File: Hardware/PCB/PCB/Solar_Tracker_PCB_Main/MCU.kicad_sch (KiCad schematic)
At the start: 16 parts, among them IC1 ESP32-S3-WROOM-1-N4R8, IC5 LM1117MPX-3.3_NOPB, J2 USB4940-00-A, J3 1729076, J4 1977223-1, J5 1977223-1

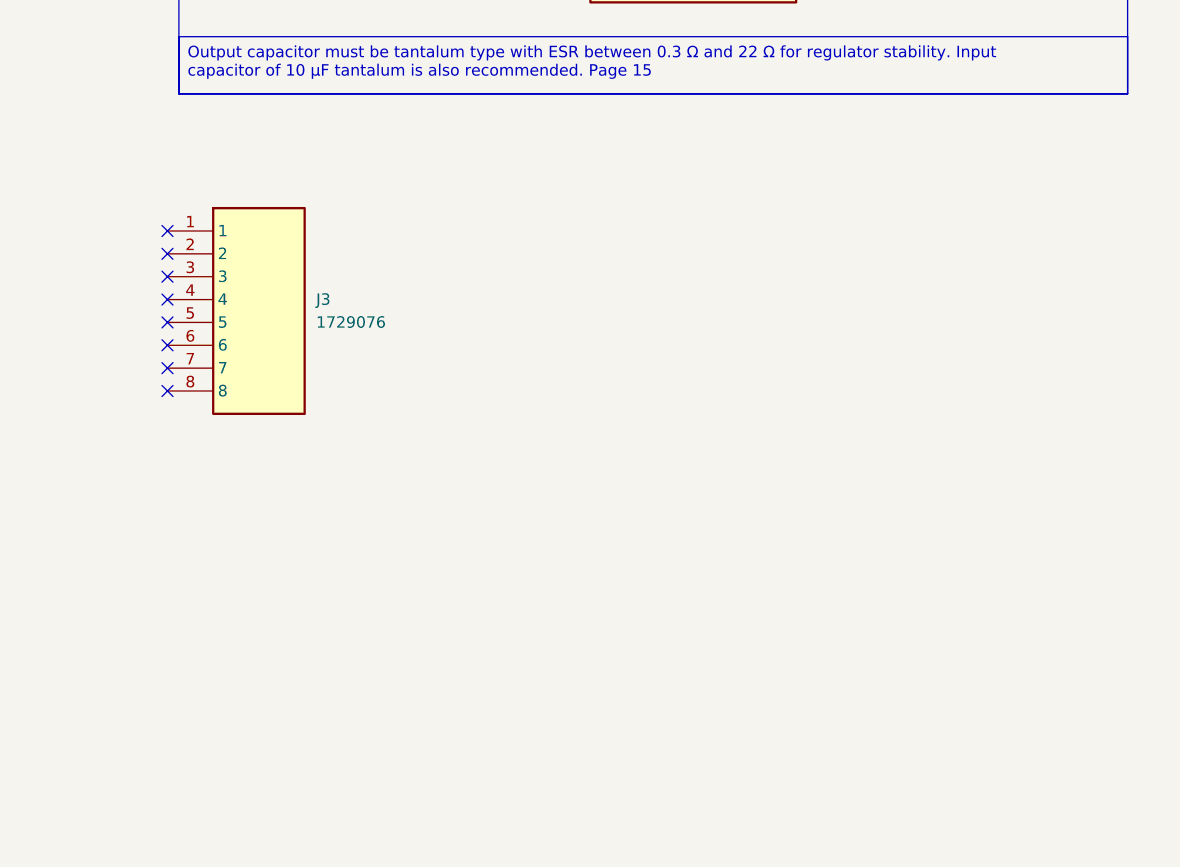
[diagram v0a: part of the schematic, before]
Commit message: Bornera
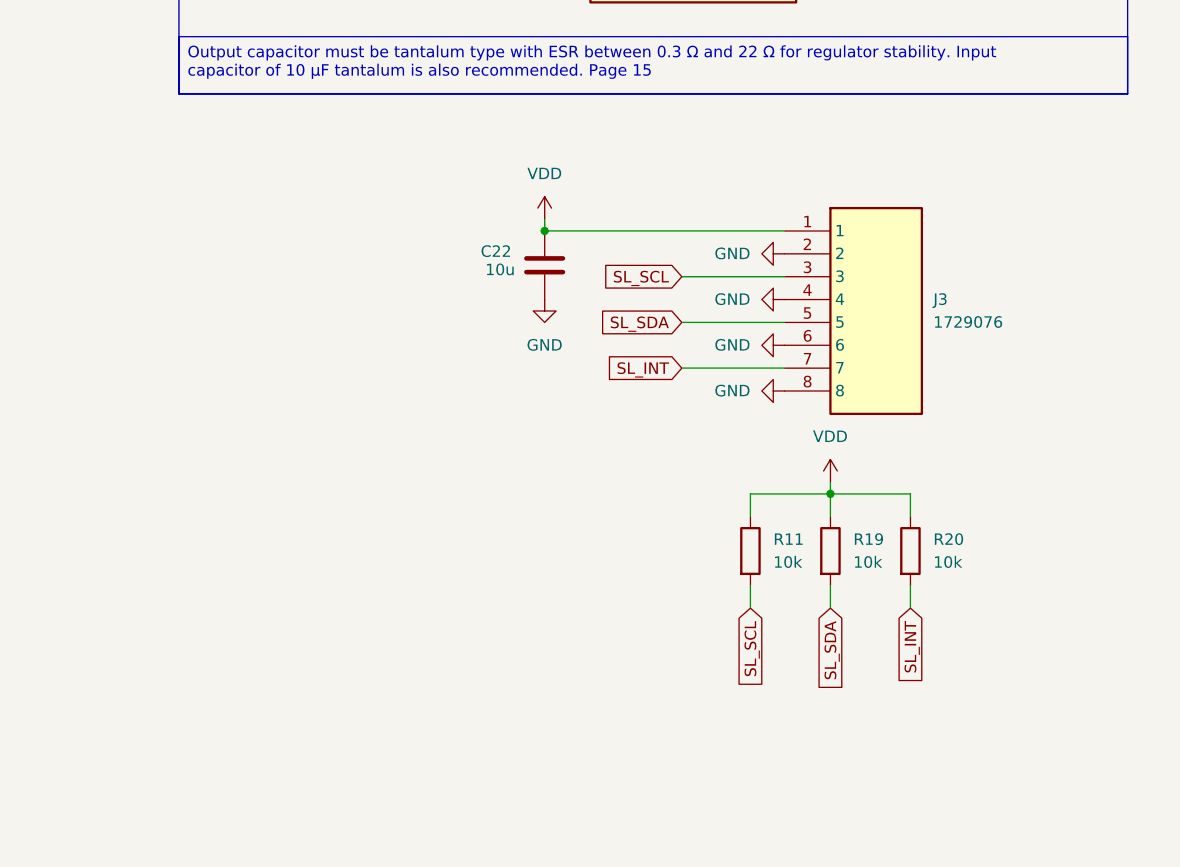
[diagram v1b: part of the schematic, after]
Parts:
- added C22: 10u, Capacitor_SMD:C_0805_2012Metric_Pad1.18x1.45mm_HandSolder, symbol Device:C
- added R11, R19, R20: 10k, Resistor_SMD:R_0805_2012Metric_Pad1.20x1.40mm_HandSolder, symbol Device:R
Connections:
- net GND: now also J3.2, J3.4, J3.6, J3.8, C22.2
- net VDD: now also J3.1, C22.1, R11.1, R19.1, R20.1
- net SL_SCL: now reaches J3.3
- net SL_SCL: now also R11.2
- net SL_SDA: now reaches J3.5
- net SL_SDA: now also R19.2
- net SL_INT: now reaches J3.7
- net SL_INT: now also R20.2
- no-connect marks 36 -> 28
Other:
- moved on the sheet: J3
